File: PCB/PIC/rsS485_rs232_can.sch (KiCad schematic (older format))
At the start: 48 parts, among them J2 TB_1X3, J3 DB9, J4 TB_1X3, U5 MAX3072, U6 ST3232E, U7 VP231, U8 PESD1CAN

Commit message: rev02 aignacion footprint
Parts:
- U5: footprint SOIC8 -> SMD_Packages:SOIC-8-N
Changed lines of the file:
@@
 F 0 "U5" H 3500 8050 30  0000 C CNN
 F 1 "MAX3072" H 3900 7550 39  0000 C CNN
-F 2 "SOIC8" H 3900 8050 35  0001 C CIN
+F 2 "SMD_Packages:SOIC-8-N" H 3900 8050 35  0001 C CIN
 F 3 "http://www.digikey.com/product-detail/en/maxim-integrated/MAX3072EESA-T/MAX3072EESA-TCT-ND/3647905" H 4350 9000 60  0001 C CNN
 	1    3700 7800

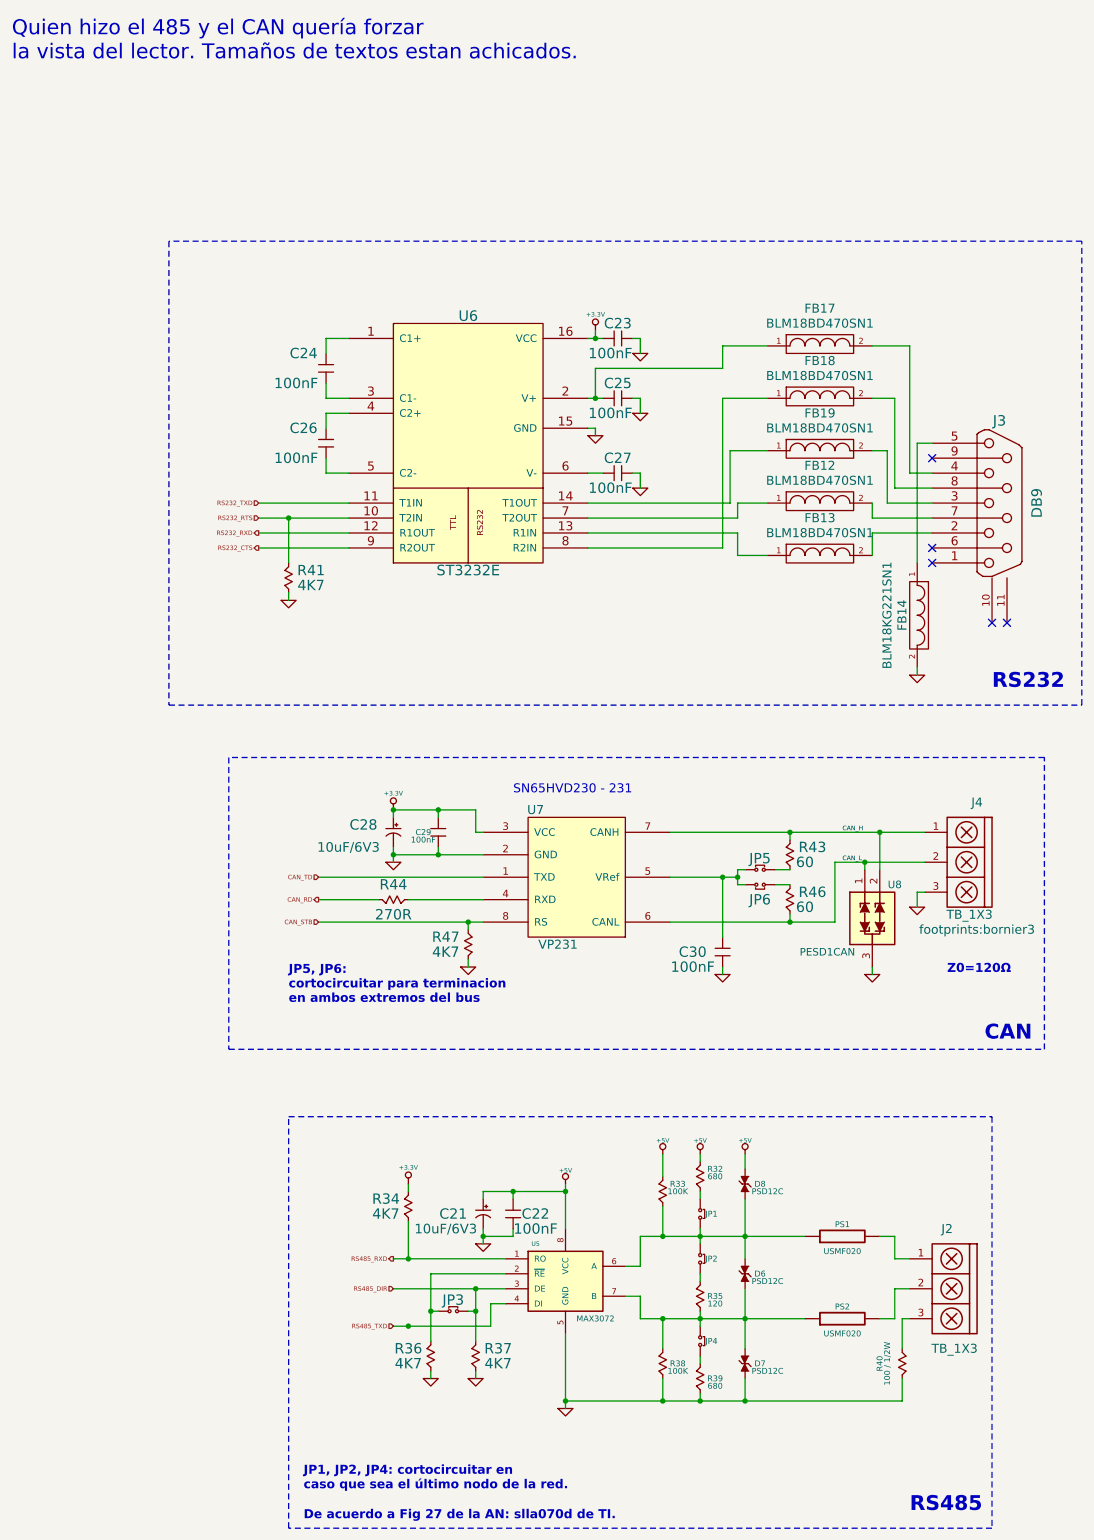
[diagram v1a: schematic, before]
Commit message: rev.02 CIAA-PIC
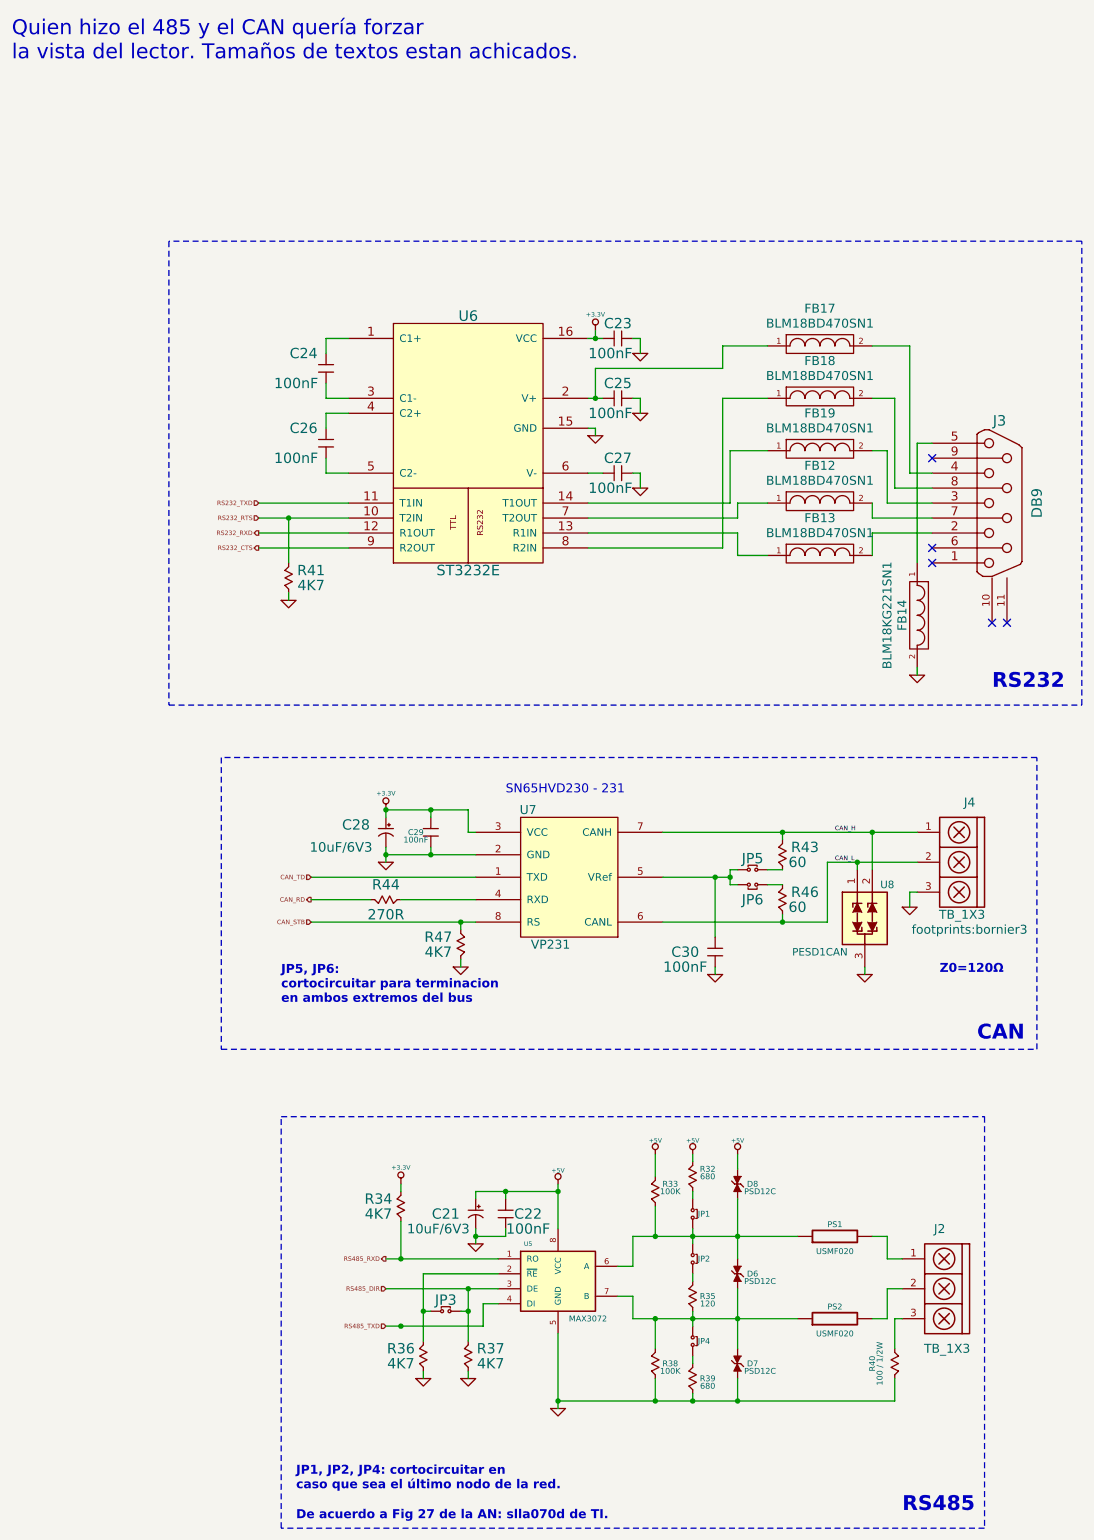
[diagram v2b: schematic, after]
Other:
- moved on the sheet: C21, C22, C28, C29, C30, D6, D7, D8, J2, J4, JP1, JP2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
